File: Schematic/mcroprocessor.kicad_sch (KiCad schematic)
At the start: 17 parts, among them J3 Conn_01x03_Pin, J3 DEBUG_HEADER, SW1 RESET, U1 STM32F091RCT6, U6 MAX7375AXR805

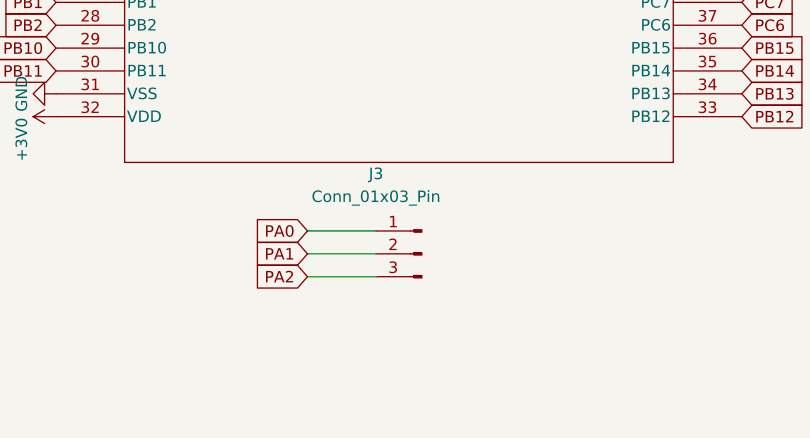
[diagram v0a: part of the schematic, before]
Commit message: Added level shifter (may or may not use) other minor fixes
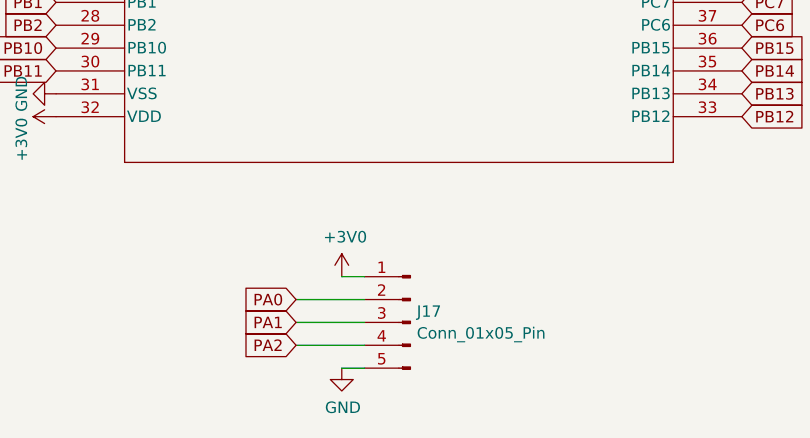
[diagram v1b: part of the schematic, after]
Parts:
- removed J3: Conn_01x03_Pin, Connector_PinSocket_2.54mm:PinSocket_1x03_P2.54mm_Vertical, symbol Connector:Conn_01x03_Pin
- added J17: Conn_01x05_Pin, Connector_PinHeader_2.54mm:PinHeader_1x05_P2.54mm_Vertical, symbol Connector:Conn_01x05_Pin
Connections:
- net +3V0: now also J17.1 (Pin_1)
- net GND: now also J17.5 (Pin_5)
- net PA0: now also J17.2 (Pin_2)
- net PA1: now also J17.3 (Pin_3)
- net PA2: now also J17.4 (Pin_4)
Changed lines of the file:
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@@
     (stroke (width 0) (type default))
   )
-  (wire (pts (xy 106.68 133.35) (xy 114.3 133.35))
+  (wire (pts (xy 105.41 140.97) (xy 113.03 140.97))
     (stroke (width 0) (type default))
   )
@@
     (stroke (width 0) (type default))
   )
+  (wire (pts (xy 110.49 143.51) (xy 113.03 143.51))
+    (stroke (width 0) (type default))
+  )
   (wire (pts (xy 238.76 129.54) (xy 241.3 129.54))
     (stroke (width 0) (type default))
@@
     (stroke (width 0) (type default))
   )
-  (wire (pts (xy 106.68 130.81) (xy 114.3 130.81))
+  (wire (pts (xy 105.41 138.43) (xy 113.03 138.43))
     (stroke (width 0) (type default))
   )
@@
     (stroke (width 0) (type default))
   )
+  (wire (pts (xy 110.49 133.35) (xy 113.03 133.35))
+    (stroke (width 0) (type default))
+  )
   (wire (pts (xy 210.82 137.16) (xy 217.17 137.16))
     (stroke (width 0) (type default))
   )
-  (wire (pts (xy 106.68 128.27) (xy 114.3 128.27))
+  (wire (pts (xy 105.41 135.89) (xy 113.03 135.89))
     (stroke (width 0) (type default))
   )
@@
     )
   )
-  (global_label "PA0" (shape input) (at 106.68 128.27 180) (fields_autoplaced)
-    (effects (font (size 1.27 1.27)) (justify right))
-    (property "Intersheetrefs" "${INTERSHEET_REFS}" (at 100.2061 128.27 0)
+  (global_label "PA0" (shape input) (at 105.41 135.89 180) (fields_autoplaced)
+    (effects (font (size 1.27 1.27)) (justify right))
+    (property "Intersheetrefs" "${INTERSHEET_REFS}" (at 98.9361 135.89 0)
       (effects (font (size 1.27 1.27)) (justify right) hide)
     )
@@
     )
   )
-  (global_label "PA2" (shape input) (at 106.68 133.35 180) (fields_autoplaced)
-    (effects (font (size 1.27 1.27)) (justify right))
-    (property "Intersheetrefs" "${INTERSHEET_REFS}" (at 100.2061 133.35 0)
+  (global_label "PA2" (shape input) (at 105.41 140.97 180) (fields_autoplaced)
+    (effects (font (size 1.27 1.27)) (justify right))
+    (property "Intersheetrefs" "${INTERSHEET_REFS}" (at 98.9361 140.97 0)
       (effects (font (size 1.27 1.27)) (justify right) hide)
     )
@@
     )
   )
-  (global_label "PA1" (shape input) (at 106.68 130.81 180) (fields_autoplaced)
-    (effects (font (size 1.27 1.27)) (justify right))
-    (property "Intersheetrefs" "${INTERSHEET_REFS}" (at 100.2061 130.81 0)
+  (global_label "PA1" (shape input) (at 105.41 138.43 180) (fields_autoplaced)
+    (effects (font (size 1.27 1.27)) (justify right))
+    (property "Intersheetrefs" "${INTERSHEET_REFS}" (at 98.9361 138.43 0)
       (effects (font (size 1.27 1.27)) (justify right) hide)
     )
@@
     )
   )
+  (symbol (lib_id "Connector:Conn_01x05_Pin") (at 118.11 138.43 0) (mirror y) (unit 1)
+    (in_bom yes) (on_board yes) (dnp no) (fields_autoplaced)
+    (property "Reference" "J17" (at 118.8212 137.2179 0)
+      (effects (font (size 1.27 1.27)) (justify right))
+    )
+    (property "Value" "Conn_01x05_Pin" (at 118.8212 139.6421 0)
+      (effects (font (size 1.27 1.27)) (justify right))
+    )
+    (property "Footprint" "Connector_PinHeader_2.54mm:PinHeader_1x05_P2.54mm_Vertical" (at 118.11 138.43 0)
+      (effects (font (size 1.27 1.27)) hide)
+    )
+    (property "Datasheet" "~" (at 118.11 138.43 0)
+      (effects (font (size 1.27 1.27)) hide)
+    )
+    (pin "1")
+    (pin "2")
+    (pin "3")
+    (pin "4")
+    (pin "5")
+    (instances
+      (project "Schematic"
+        (path "/ced54cd9-3b34-40e4-aa66-964aaab81b0a/49528601-a054-44d2-8cd6-b055d7d9a1ef"
+          (reference "J17") (unit 1)
+        )
+      )
+    )
+  )
   (symbol (lib_id "power:+3V0") (at 154.94 77.47 270) (unit 1)
     (in_bom yes) (on_board yes) (dnp no)
@@
         (path "/ced54cd9-3b34-40e4-aa66-964aaab81b0a/575551e4-af3a-490e-80f8-c842b6f0dfe5"
           (reference "#PWR024") (unit 1)
-        )
-      )
-    )
-  )
-  (symbol (lib_id "Connector:Conn_01x03_Pin") (at 119.38 130.81 0) (mirror y) (unit 1)
-    (in_bom yes) (on_board yes) (dnp no)
-    (property "Reference" "J3" (at 114.3 121.92 0)
-      (effects (font (size 1.27 1.27)))
-    )
-    (property "Value" "Conn_01x03_Pin" (at 114.3 124.46 0)
-      (effects (font (size 1.27 1.27)))
-    )
-    (property "Footprint" "Connector_PinSocket_2.54mm:PinSocket_1x03_P2.54mm_Vertical" (at 119.38 130.81 0)
-      (effects (font (size 1.27 1.27)) hide)
-    )
-    (property "Datasheet" "~" (at 119.38 130.81 0)
-      (effects (font (size 1.27 1.27)) hide)
-    )
-    (pin "1")
-    (pin "2")
-    (pin "3")
-    (instances
-      (project "LM2678 - 5.0V"
-        (path "/519fb26c-708f-40e5-b123-022e0171115d"
-          (reference "J3") (unit 1)
-        )
-      )
-      (project "Schematic"
-        (path "/ced54cd9-3b34-40e4-aa66-964aaab81b0a/17b7dae5-2f82-4d17-9b49-7ea60414647f"
-          (reference "J6") (unit 1)
-        )
-        (path "/ced54cd9-3b34-40e4-aa66-964aaab81b0a/49528601-a054-44d2-8cd6-b055d7d9a1ef"
-          (reference "J17") (unit 1)
         )
       )
@@
         )
       )
+    )
+  )
+  (symbol (lib_id "power:GND") (at 110.49 143.51 0) (unit 1)
+    (in_bom yes) (on_board yes) (dnp no)
+    (property "Reference" "#PWR0130" (at 110.49 149.86 0)
+      (effects (font (size 1.27 1.27)) hide)
+    )
+    (property "Value" "GND" (at 110.617 147.9042 0)
+      (effects (font (size 1.27 1.27)))
+    )
+    (property "Footprint" "" (at 110.49 143.51 0)
+      (effects (font (size 1.27 1.27)) hide)
+    )
+    (property "Datasheet" "" (at 110.49 143.51 0)
+      (effects (font (size 1.27 1.27)) hide)
+    )
+    (pin "1")
+    (instances
+      (project "stm32f091"
+        (path "/1a854c3f-f20e-4271-9c06-678b7140bb2e"
+          (reference "#PWR0130") (unit 1)
+        )
+      )
+      (project "Schematic"
+        (path "/ced54cd9-3b34-40e4-aa66-964aaab81b0a/49528601-a054-44d2-8cd6-b055d7d9a1ef"
+          (reference "#PWR089") (unit 1)
+        )
+        (path "/ced54cd9-3b34-40e4-aa66-964aaab81b0a"
+          (reference "#PWR019") (unit 1)
+        )
+        (path "/ced54cd9-3b34-40e4-aa66-964aaab81b0a/1629468b-8e9d-4ab7-97ca-858e6989be67"
+          (reference "#PWR024") (unit 1)
+        )
+        (path "/ced54cd9-3b34-40e4-aa66-964aaab81b0a/575551e4-af3a-490e-80f8-c842b6f0dfe5"
+          (reference "#PWR024") (unit 1)
+        )
+      )
+    )
+  )
+  (symbol (lib_id "power:+3V0") (at 110.49 133.35 0) (unit 1)
+    (in_bom yes) (on_board yes) (dnp no)
+    (property "Reference" "#PWR0104" (at 110.49 137.16 0)
+      (effects (font (size 1.27 1.27)) hide)
+    )
+    (property "Value" "+3V0" (at 110.871 128.9558 0)
+      (effects (font (size 1.27 1.27)))
+    )
+    (property "Footprint" "" (at 110.49 133.35 0)
+      (effects (font (size 1.27 1.27)) hide)
+    )
+    (property "Datasheet" "" (at 110.49 133.35 0)
+      (effects (font (size 1.27 1.27)) hide)
+    )
+    (pin "1")
+    (instances
+      (project "stm32f091"
+        (path "/1a854c3f-f20e-4271-9c06-678b7140bb2e"
+          (reference "#PWR0104") (unit 1)
+        )
+      )
+      (project "Schematic"
+        (path "/ced54cd9-3b34-40e4-aa66-964aaab81b0a/49528601-a054-44d2-8cd6-b055d7d9a1ef"
+          (reference "#PWR088") (unit 1)
+        )
+      )
